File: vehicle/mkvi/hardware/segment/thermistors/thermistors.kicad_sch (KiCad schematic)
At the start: 1 part, among them J1 TST-108-01-T-D

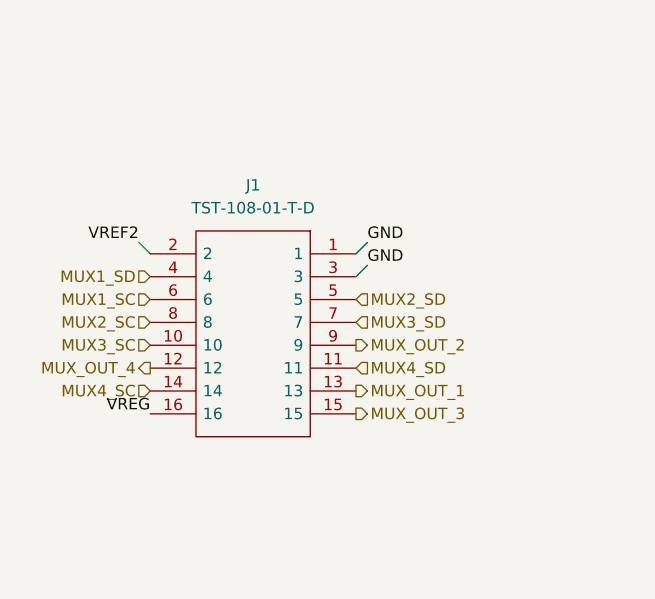
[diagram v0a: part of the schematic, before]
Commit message: merge main //vehicle
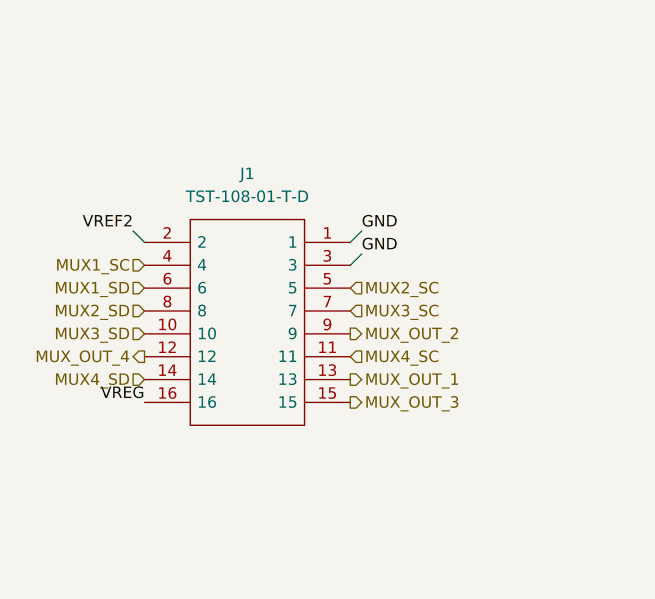
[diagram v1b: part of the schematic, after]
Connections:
- net MUX1_SC: now also J1.4; no longer J1.6
- net MUX1_SD: now also J1.6; no longer J1.4
- net MUX2_SC: now also J1.5; no longer J1.8
- net MUX2_SD: now also J1.8; no longer J1.5
- net MUX3_SC: now also J1.7; no longer J1.10
- net MUX3_SD: now also J1.10; no longer J1.7
- net MUX4_SC: now also J1.11; no longer J1.14
- net MUX4_SD: now also J1.14; no longer J1.11
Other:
- moved on the sheet: J1
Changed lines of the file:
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@@
 (kicad_sch (version 20230121) (generator eeschema)
   (paper "A4")
-  (wire (pts (xy 64.135 62.23) (xy 62.865 63.5))
+  (wire (pts (xy 63.5 60.96) (xy 62.23 62.23))
     (stroke (width 0) (type default))
   )
-  (wire (pts (xy 38.735 59.69) (xy 40.005 60.96))
+  (wire (pts (xy 38.1 58.42) (xy 39.37 59.69))
     (stroke (width 0) (type default))
   )
@@
     (stroke (width 0) (type default))
   )
-  (wire (pts (xy 64.135 59.69) (xy 62.865 60.96))
+  (wire (pts (xy 63.5 58.42) (xy 62.23 59.69))
     (stroke (width 0) (type default))
   )
@@
     (effects (font (size 1.27 1.27)) (justify right bottom))
   )
-  (label "VREG" (at 40.005 78.74 180) (fields_autoplaced)
+  (label "VREG" (at 39.37 77.47 180) (fields_autoplaced)
     (effects (font (size 1.27 1.27)) (justify right bottom))
   )
@@
     (effects (font (size 1.27 1.27)) (justify right bottom))
   )
-  (label "VREF2" (at 38.735 59.69 180) (fields_autoplaced)
+  (label "VREF2" (at 38.1 58.42 180) (fields_autoplaced)
     (effects (font (size 1.27 1.27)) (justify right bottom))
   )
@@
     (effects (font (size 1.27 1.27)) (justify left bottom))
   )
-  (label "GND" (at 64.135 59.69 0) (fields_autoplaced)
+  (label "GND" (at 63.5 58.42 0) (fields_autoplaced)
     (effects (font (size 1.27 1.27)) (justify left bottom))
   )
@@
     (effects (font (size 1.27 1.27)) (justify right bottom))
   )
-  (label "GND" (at 64.135 62.23 0) (fields_autoplaced)
+  (label "GND" (at 63.5 60.96 0) (fields_autoplaced)
     (effects (font (size 1.27 1.27)) (justify left bottom))
   )
@@
     (effects (font (size 1.27 1.27)) (justify left))
   )
-  (hierarchical_label "MUX_OUT_3" (shape output) (at 62.865 78.74 0) (fields_autoplaced)
+  (hierarchical_label "MUX2_SC" (shape input) (at 62.23 64.77 0) (fields_autoplaced)
+    (effects (font (size 1.27 1.27)) (justify left))
+  )
+  (hierarchical_label "MUX_OUT_3" (shape output) (at 62.23 77.47 0) (fields_autoplaced)
     (effects (font (size 1.27 1.27)) (justify left))
   )
@@
     (effects (font (size 1.27 1.27)) (justify left))
   )
-  (hierarchical_label "MUX3_SC" (shape input) (at 40.005 71.12 180) (fields_autoplaced)
+  (hierarchical_label "MUX1_SD" (shape input) (at 39.37 64.77 180) (fields_autoplaced)
     (effects (font (size 1.27 1.27)) (justify right))
-  )
-  (hierarchical_label "MUX3_SD" (shape input) (at 62.865 68.58 0) (fields_autoplaced)
-    (effects (font (size 1.27 1.27)) (justify left))
   )
   (hierarchical_label "MUX4_SD" (shape input) (at 235.585 136.525 0) (fields_autoplaced)
     (effects (font (size 1.27 1.27)) (justify left))
   )
-  (hierarchical_label "MUX1_SD" (shape input) (at 40.005 63.5 180) (fields_autoplaced)
+  (hierarchical_label "MUX4_SD" (shape input) (at 39.37 74.93 180) (fields_autoplaced)
     (effects (font (size 1.27 1.27)) (justify right))
   )
-  (hierarchical_label "MUX4_SC" (shape input) (at 40.005 76.2 180) (fields_autoplaced)
-    (effects (font (size 1.27 1.27)) (justify right))
-  )
-  (hierarchical_label "MUX2_SD" (shape input) (at 62.865 66.04 0) (fields_autoplaced)
+  (hierarchical_label "MUX3_SD" (shape input) (at 235.585 100.965 0) (fields_autoplaced)
     (effects (font (size 1.27 1.27)) (justify left))
   )
-  (hierarchical_label "MUX3_SD" (shape input) (at 235.585 100.965 0) (fields_autoplaced)
+  (hierarchical_label "MUX3_SC" (shape input) (at 62.23 67.31 0) (fields_autoplaced)
     (effects (font (size 1.27 1.27)) (justify left))
   )
@@
     (effects (font (size 1.27 1.27)) (justify left))
   )
-  (hierarchical_label "MUX_OUT_1" (shape output) (at 62.865 76.2 0) (fields_autoplaced)
+  (hierarchical_label "MUX4_SC" (shape input) (at 62.23 72.39 0) (fields_autoplaced)
+    (effects (font (size 1.27 1.27)) (justify left))
+  )
+  (hierarchical_label "MUX_OUT_1" (shape output) (at 62.23 74.93 0) (fields_autoplaced)
     (effects (font (size 1.27 1.27)) (justify left))
   )
   (hierarchical_label "MUX2_SD" (shape input) (at 234.315 63.5 0) (fields_autoplaced)
-    (effects (font (size 1.27 1.27)) (justify left))
-  )
-  (hierarchical_label "MUX4_SD" (shape input) (at 62.865 73.66 0) (fields_autoplaced)
     (effects (font (size 1.27 1.27)) (justify left))
   )
@@
     (effects (font (size 1.27 1.27)) (justify left))
   )
-  (hierarchical_label "MUX1_SC" (shape input) (at 40.005 66.04 180) (fields_autoplaced)
+  (hierarchical_label "MUX3_SD" (shape input) (at 39.37 69.85 180) (fields_autoplaced)
     (effects (font (size 1.27 1.27)) (justify right))
   )
-  (hierarchical_label "MUX_OUT_2" (shape output) (at 62.865 71.12 0) (fields_autoplaced)
+  (hierarchical_label "MUX_OUT_2" (shape output) (at 62.23 69.85 0) (fields_autoplaced)
     (effects (font (size 1.27 1.27)) (justify left))
   )
-  (hierarchical_label "MUX_OUT_4" (shape output) (at 40.005 73.66 180) (fields_autoplaced)
+  (hierarchical_label "MUX_OUT_4" (shape output) (at 39.37 72.39 180) (fields_autoplaced)
     (effects (font (size 1.27 1.27)) (justify right))
   )
@@
     (effects (font (size 1.27 1.27)) (justify left))
   )
-  (hierarchical_label "MUX2_SC" (shape input) (at 40.005 68.58 180) (fields_autoplaced)
+  (hierarchical_label "MUX1_SC" (shape input) (at 39.37 62.23 180) (fields_autoplaced)
     (effects (font (size 1.27 1.27)) (justify right))
   )
@@
     (effects (font (size 1.27 1.27)) (justify left))
   )
-  (symbol (lib_id "OEM:TST-108-01-T-D") (at 51.435 69.85 0) (mirror y) (unit 1)
+  (hierarchical_label "MUX2_SD" (shape input) (at 39.37 67.31 180) (fields_autoplaced)
+    (effects (font (size 1.27 1.27)) (justify right))
+  )
+  (symbol (lib_id "OEM:TST-108-01-T-D") (at 50.8 68.58 0) (mirror y) (unit 1)
     (in_bom yes) (on_board yes) (dnp no) (fields_autoplaced)
-    (property "Reference" "J1" (at 51.435 53.34 0)
+    (property "Reference" "J1" (at 50.8 52.07 0)
       (effects (font (size 1.27 1.27)))
     )
-    (property "Value" "TST-108-01-T-D" (at 51.435 55.88 0)
+    (property "Value" "TST-108-01-T-D" (at 50.8 54.61 0)
       (effects (font (size 1.27 1.27)))
     )
-    (property "Footprint" "OEM:TST-108-XX-T-D" (at 43.815 58.42 0)
+    (property "Footprint" "OEM:TST-108-XX-T-D" (at 43.18 57.15 0)
       (effects (font (size 1.27 1.27)) (justify left) hide)
     )
-    (property "Datasheet" "http://suddendocs.samtec.com/prints/tst-1xx-xx-x-x-xx-xx-mkt.pdf" (at 32.385 69.85 0)
+    (property "Datasheet" "http://suddendocs.samtec.com/prints/tst-1xx-xx-x-x-xx-xx-mkt.pdf" (at 31.75 68.58 0)
       (effects (font (size 1.27 1.27)) (justify left) hide)
     )
-    (property "MPN" "TST-108-01-T-D" (at 43.815 76.2 0)
+    (property "MPN" "TST-108-01-T-D" (at 43.18 74.93 0)
       (effects (font (size 1.27 1.27)) (justify left) hide)
     )
-    (property "MFN" "Samtec" (at 51.435 69.85 0)
+    (property "MFN" "Samtec" (at 50.8 68.58 0)
       (effects (font (size 1.27 1.27)) hide)
     )
-    (property "DKPN" "SAM13026-ND" (at 51.435 69.85 0)
+    (property "DKPN" "SAM13026-ND" (at 50.8 68.58 0)
       (effects (font (size 1.27 1.27)) hide)
     )
-    (property "NewDesigns" "YES" (at 51.435 69.85 0)
+    (property "NewDesigns" "YES" (at 50.8 68.58 0)
       (effects (font (size 1.27 1.27)) hide)
     )
-    (property "Stocked" "Bulk" (at 51.435 69.85 0)
+    (property "Stocked" "Bulk" (at 50.8 68.58 0)
       (effects (font (size 1.27 1.27)) hide)
     )
-    (property "Package" "Custom" (at 51.435 69.85 0)
+    (property "Package" "Custom" (at 50.8 68.58 0)
       (effects (font (size 1.27 1.27)) hide)
     )
-    (property "Style" "THT" (at 51.435 69.85 0)
+    (property "Style" "THT" (at 50.8 68.58 0)
       (effects (font (size 1.27 1.27)) hide)
     )
-    (property "MatesWith" "IDSD-08-D-04.00-T-G-ND" (at 51.435 69.85 0)
+    (property "MatesWith" "IDSD-08-D-04.00-T-G-ND" (at 50.8 68.58 0)
       (effects (font (size 1.27 1.27)) hide)
     )
